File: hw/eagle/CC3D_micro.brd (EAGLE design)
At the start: 29.7 x 19.3 mm, 76 parts, among them IC1 STM32F103CBT6, IC2 MPU-6050, IC3 MS5611, IC4 SPI_FLASH-X25XXSMD, IC5 MCP1703CB, U2 STM32F030XTSSOP20, Y1 8MHZ

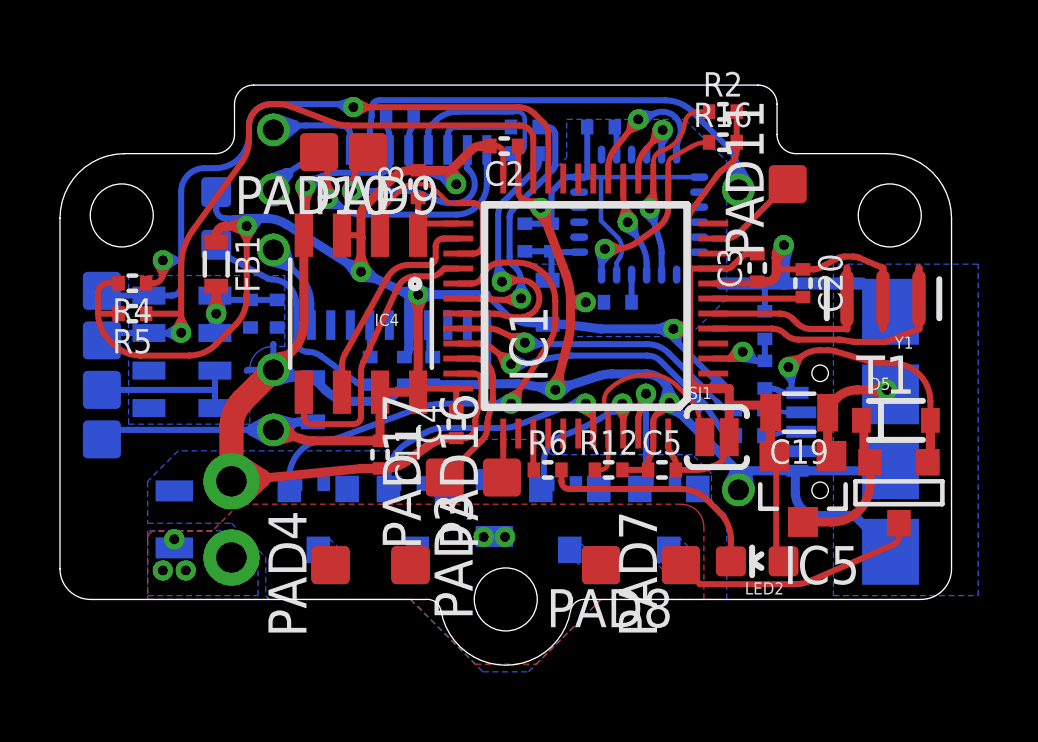
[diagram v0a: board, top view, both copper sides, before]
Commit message: hw v0.2
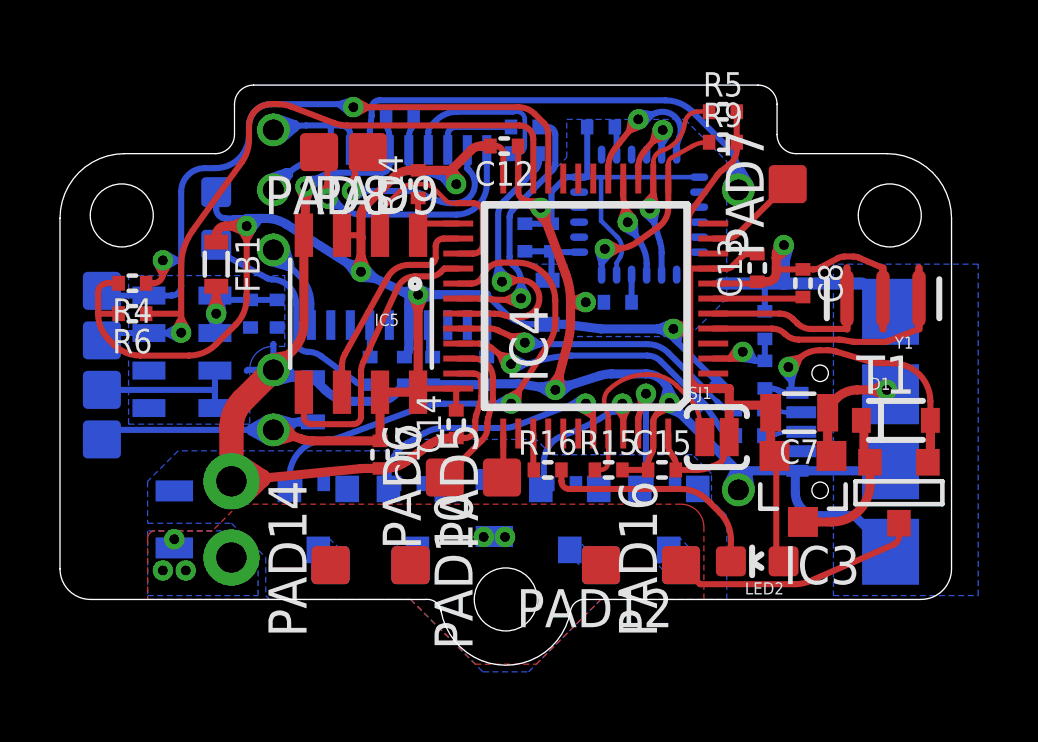
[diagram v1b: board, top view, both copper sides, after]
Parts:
- removed C20: 47n, RC.v2:0402
- added C1: u47, RC.v2:0402
- added R1: 22, RC.v2:0402
- C10: value 47n -> u1
- C11, C3: value 0u1 -> 47n
- C12: device RC.v2:0603 -> RC.v2:0402
- C13, C14: value 2u2 -> 0u1; device RC.v2:0805 -> RC.v2:0402
- C16: value 47n -> 0u1; device RC.v2:0402 -> RC.v2:0603
- C17: value 2n2 50v -> 0u1
- C18: value u47 -> 2u2; device RC.v2:0402 -> RC.v2:0805
- C19: value u47 -> 2u2
- C2: value 0u1 -> u47
- C5: value 0u1 -> 2n2 50v
- C6: value u1 -> 47n
- C7: value u1 -> u47; device RC.v2:0402 -> RC.v2:0805
- C9: value u47 -> u1
- IC1: value STM32F103CBT6 -> MPU-6050; device cc3d:LQFP48 -> cc3d:QFN-24-TESTING
- IC2: value MPU-6050 -> MS5611; device cc3d:QFN-24-TESTING -> cc3d:LGA8
- IC3: value MS5611 -> MCP1703CB; device cc3d:LGA8 -> semi:SOT23
- IC4: value SPI_FLASH-X25XXSMD -> STM32F103CBT6; device cc3d:SO08 -> cc3d:LQFP48
- IC5: value MCP1703CB -> SPI_FLASH-X25XXSMD; device semi:SOT23 -> cc3d:SO08
- IC6: value STM32F030XTSSOP20 -> STM32F030F4T6
- PAD1: value (none) -> VCC
- PAD10, PAD16: value SWCLK -> (none)
- PAD11: value PPM -> (none)
- PAD12: value RX/SDA -> (none)
- PAD13: value TX/SCL -> (none)
- PAD14: value VCC -> (none)
- PAD15: value GND -> (none)
- PAD17: value SWDIO -> (none)
- PAD2: value (none) -> GND
- PAD3: value (none) -> RX/SDA
- PAD4: value (none) -> TX/SCL
- PAD5, PAD8: value (none) -> SWCLK
- PAD6: value (none) -> SWDIO
- PAD7: value (none) -> PPM
- R10: value 10k -> 1k
- R11: value 15k -> 680
- R12: value 1k -> 510
- R14: value 510 -> 10k
- R15: value 680 -> 1k
- R16: value DNP -> 680
- R2: value 10k -> 22
- R3: value 10k -> 1k5
- R5: value 2k2 -> 10k
- R6: value 680 -> 2k2
- R7: value 22 -> 10k
- R8: value 22 -> 15k
- R9: value 1k5 -> DNP
- moved IC3 21.2 mm to (9.91, 3.68), flipped to the top, turned to 180 degrees
- moved R5 20.8 mm to (7.24, 16.3), turned to 0 degrees
- moved PAD1 19.8 mm to (-13.5, 5.33), turned to 90 degrees
- moved PAD12 18.2 mm to (3.17, 1.14), flipped to the top
- moved PAD15 17.6 mm to (3.17, 1.14), turned to 0 degrees
- moved PAD2 17.6 mm to (-13.5, 6.99), turned to 90 degrees
- moved PAD8 16.7 mm to (-6.22, 14.9)
- moved C7 16.6 mm to (9.78, 6.22), flipped to the top, turned to 180 degrees
- moved IC2 15.9 mm to (-10.8, 8.26)
- moved IC5 15.8 mm to (-4.83, 9.53)
- moved C18 15.7 mm to (-11.0, 2.67)
- moved R6 14.8 mm to (-12.4, 9.53), turned to 180 degrees
- moved PAD10 14.1 mm to (-3.17, 1.14), turned to 180 degrees
- moved PAD13 13.8 mm to (-3.17, 1.14), turned to 180 degrees
- moved R11 13.2 mm to (-4.52, 7.62), turned to 270 degrees
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- renumbered D5 to D1, U2 to IC6
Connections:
- new net N$7: IC6.1, R10.P$1
- net BAT: now also C18.P$2, C19.P$2, PAD10.1, PAD12.1, PAD14.1, PAD16.1; no longer C13.P$2, C14.P$2, PAD3.1, PAD4.1, PAD7.1, PAD8.1
- net FLEXI_RX/SDA: now also IC2.7, IC4.22, PAD3.1, R6.P$1; no longer IC1.22, IC3.7, PAD12.1, R5.P$1
- net FLEXI_TX/SCL: now also IC2.8, IC4.21, PAD4.1; no longer IC1.21, IC3.8, PAD13.1
- net GND: now also C1.P$1, C10.P$2, C11.P$1, C12.P$1, C16.P$2, C17.P$2, C7.P$1, IC1.1, IC1.11, IC1.18, IC2.3, IC2.4, IC3.1, IC4.23, IC4.35, IC4.47, IC4.8, IC5.4, PAD2.1, R10.P$2, R15.P$2, R8.P$2; no longer C10.P$1, C11.P$2, C12.P$2, C16.P$1, C17.P$1, C20.P$1, C7.P$2, IC1.23, IC1.35, IC1.47, IC1.8, IC2.1, IC2.11, IC2.18, IC3.3, IC3.4, IC4.4, IC5.1, IC6.1, PAD15.1, R11.P$2, R12.P$2
- net M1+: now also PAD11.1; no longer PAD1.1
- net M2+: now also PAD15.1, Q3.1; no longer PAD2.1, Q2.1
- net M3+: now also PAD13.1, Q2.1; no longer PAD5.1, Q3.1
- net M4+: now also PAD17.1; no longer PAD6.1
- net MAIN_RX: now also IC4.31; no longer IC1.31
- net MAIN_TX: now also IC4.30, R12.P$2; no longer IC1.30, R14.P$2
- net N$1: now also IC1.12, IC4.13, R9.P$1; no longer IC1.13, IC2.12, R16.P$1
- net N$10: now also IC4.26, IC5.6; no longer IC1.26, IC4.6
- net N$11: now also IC4.27, IC5.2; no longer IC1.27, IC4.2
- net N$12: now also IC4.28, IC5.5; no longer IC1.28, IC4.5
- net N$13: now also IC4.6; no longer IC1.6
- net N$15: now also IC4.39, R16.P$1; no longer IC1.39, R6.P$1
- net N$16: now also R16.P$2; no longer R6.P$2
- net N$17: now also IC4.3, R7.P$2, R8.P$1; no longer IC1.3, R10.P$2, R11.P$1
- net N$18: now also R2.P$2; no longer R8.P$2
- net N$19: now also IC4.44, R15.P$1; no longer IC1.44, R12.P$1
- net N$2: now also IC1.8, IC4.14, R5.P$1; no longer IC1.14, IC2.8, R2.P$1
- net N$20: now also R1.P$2; no longer R7.P$2
- net N$24: now also R11.P$2; no longer R15.P$2
- net N$25: now also IC6.12
- net N$27: now also R12.P$1; no longer R14.P$1
- net N$3: now also IC1.23, IC4.15; no longer IC1.15, IC2.23
- net N$30: now also PAD8.1; no longer PAD10.1
- net N$31: now also R11.P$1; no longer R15.P$1
- net N$32: now also C4.P$2, IC1.10; no longer C15.P$2, IC2.10
- net N$33: now also IC4.5; no longer IC1.5
- net N$34: now also C5.P$2, IC1.20; no longer C17.P$2, IC2.20
- net N$35: now also IC4.11, PAD7.1; no longer IC1.11, PAD11.1
- net N$36: now also IC3.3; no longer IC5.3
- net N$37: now also C8.P$2, IC4.7; no longer C20.P$2, IC1.7
- net N$38: now also C11.P$2; no longer C8.P$2
- net N$4: now also IC1.9, IC4.16; no longer IC1.16, IC2.9
- net N$5: now also IC1.24, IC4.17; no longer IC1.17, IC2.24
- net N$6: now also IC4.10; no longer IC1.10
- net N$9: now also IC4.25, IC5.1, R14.P$1; no longer IC1.25, IC4.1, R3.P$1
- net PWM1: now also IC4.46; no longer IC1.46
- net PWM2: now also IC4.45, Q3.3, R19.P$2; no longer IC1.45, Q2.3, R18.P$2
- net PWM3: now also IC4.43, Q2.3, R18.P$2; no longer IC1.43, Q3.3, R19.P$2
- net PWM4: now also IC4.29; no longer IC1.29
- net SWCLK: now also IC4.37, PAD5.1; no longer IC1.37, PAD16.1
- net SWDIO: now also IC4.34, PAD6.1; no longer IC1.34, PAD17.1
- net USB_DM: now also IC4.32, R2.P$1; no longer IC1.32, R8.P$1
- net USB_DP: now also IC4.33, R1.P$1, R3.P$2; no longer IC1.33, R7.P$1, R9.P$2
- net VBUS: now also R7.P$1; no longer R10.P$1
- net VCC: now also C10.P$1, C12.P$2, C13.P$2, C14.P$2, C15.P$2, C16.P$1, C17.P$1, C7.P$2, C9.P$2, IC3.2, IC4.1, IC4.24, IC4.36, IC4.48, IC4.9, IC5.3, IC5.7, IC5.8, PAD1.1, R14.P$2, R3.P$1, R6.P$2, R9.P$2; no longer C11.P$1, C12.P$1, C19.P$2, C2.P$2, C3.P$2, C4.P$2, C5.P$2, C6.P$2, C7.P$1, IC1.1, IC1.24, IC1.36, IC1.48, IC1.9, IC4.3, IC4.7, IC4.8, IC5.2, PAD14.1, R16.P$2, R2.P$2, R3.P$2, R9.P$1
- net V_BARO: now also C1.P$2, C6.P$2, IC2.1, IC2.2; no longer C10.P$2, C9.P$2, IC3.1, IC3.2
- net V_GYRO: now also C2.P$2, C3.P$2, IC1.13; no longer C16.P$2, C18.P$2, IC2.13
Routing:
- net GND: track 139.9 -> 137.9 mm
- net N$7: track 0.00 -> 1.07 mm
- net N$25: track 5.11 -> 5.93 mm
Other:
- board text added: "BIND"
- board text added: "V0.2"
